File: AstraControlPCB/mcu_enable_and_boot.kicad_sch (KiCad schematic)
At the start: 14 parts, among them SW1 TS_Basic_Small, SW2 TS_Basic_Small

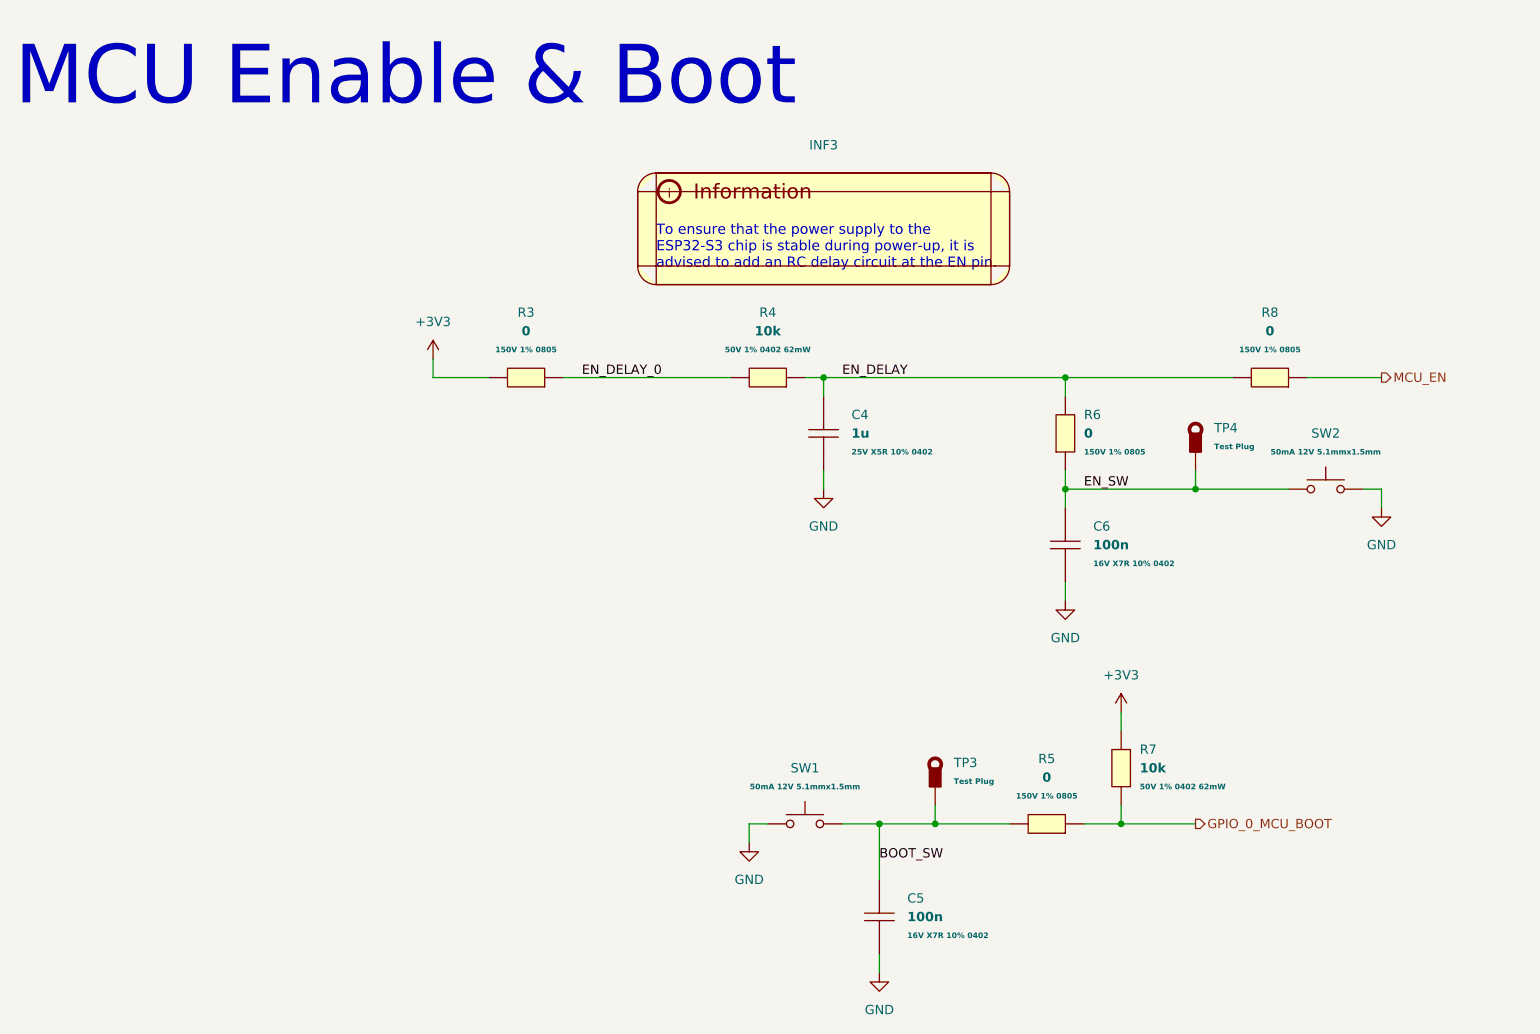
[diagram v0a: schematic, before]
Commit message: Minor cleanup
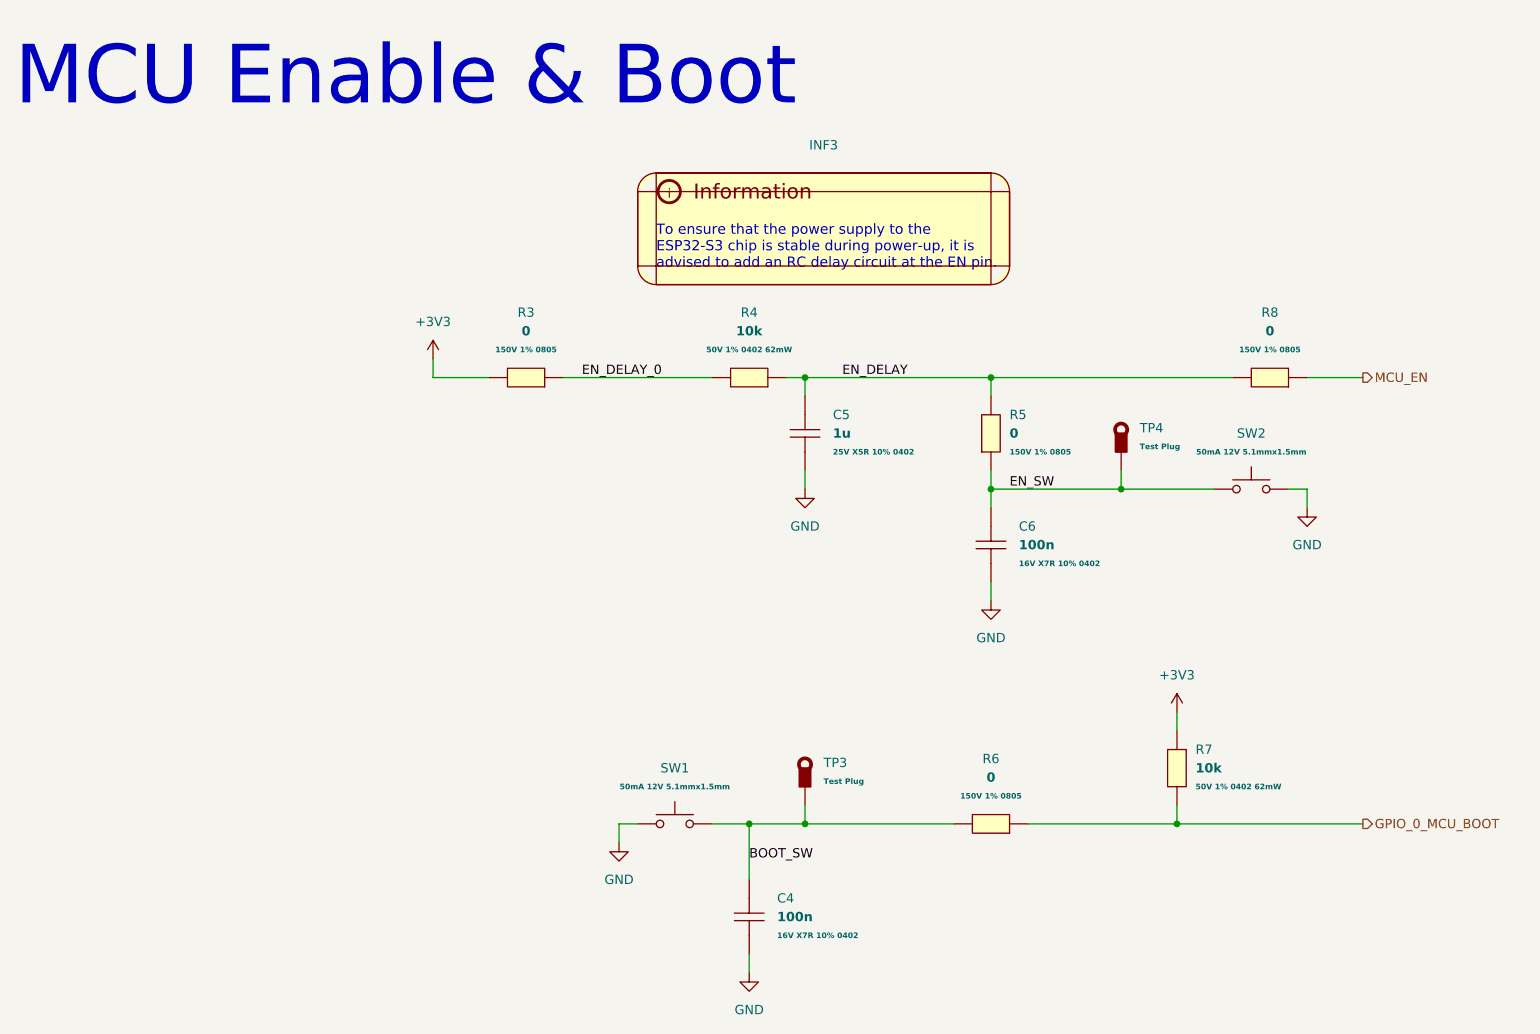
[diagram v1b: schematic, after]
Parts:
- renumbered C5 to C4, C4 to C5, R6 to R5, R5 to R6
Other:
- moved on the sheet: C4, C5, C6, R4, R5, R6, R7, SW1, SW2, TP3, TP4
